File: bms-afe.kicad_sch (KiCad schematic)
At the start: 13 parts, among them J1 CONN HEADER VERT 7POS 2.5MM

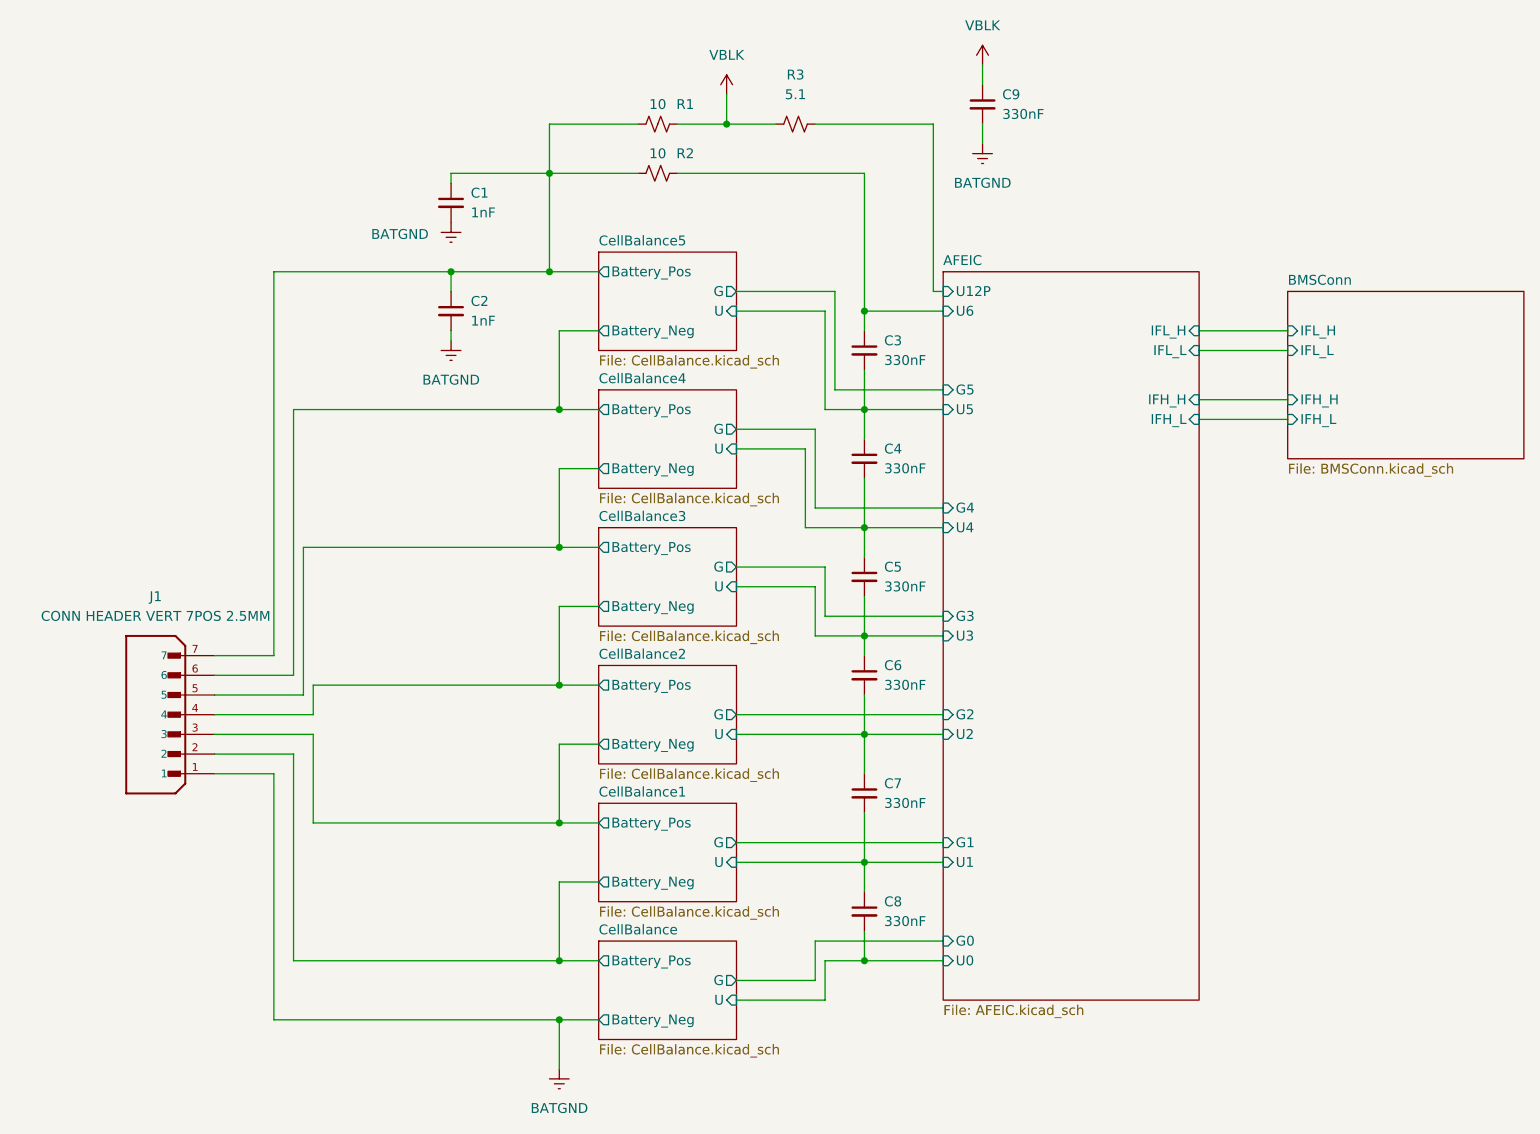
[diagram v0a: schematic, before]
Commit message: passive values
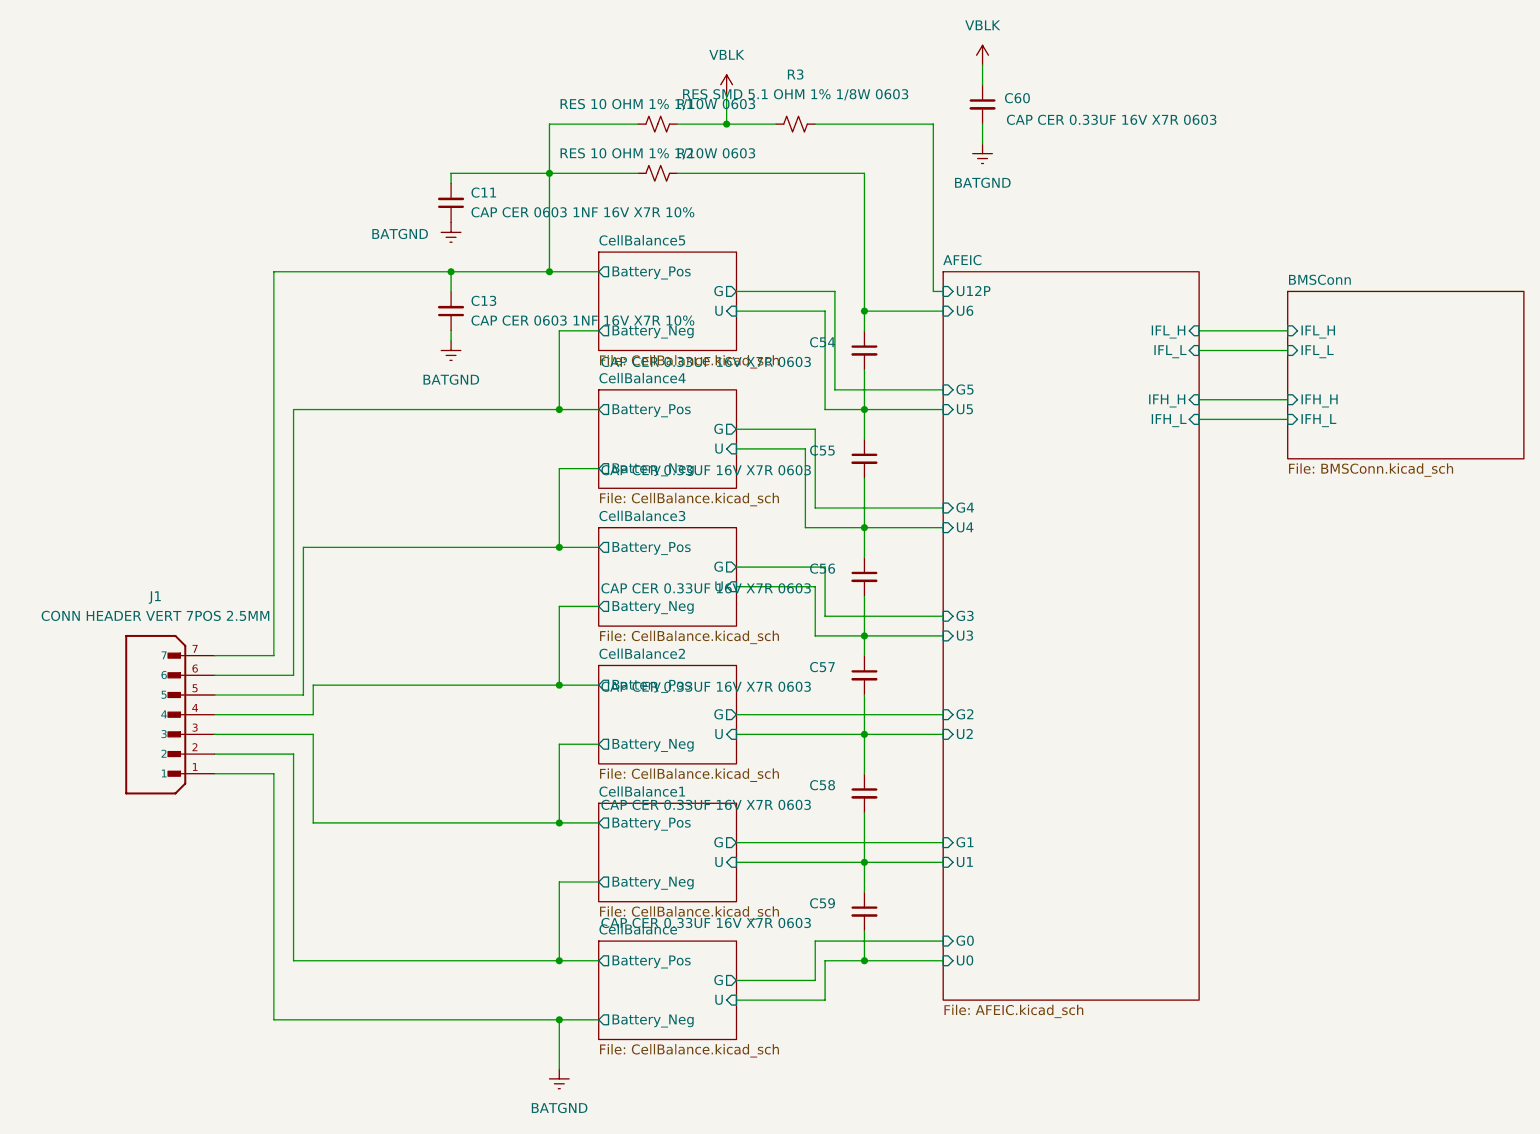
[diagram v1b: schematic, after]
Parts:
- removed C1, C2: 1nF, symbol Device:C_Small
- removed C3, C4, C5, C6, C7, C8, C9: 330nF, symbol Device:C_Small
- added C11, C13: CAP CER 0603 1NF 16V X7R 10%, Capacitor_SMD:C_0603_1608Metric, symbol Device:C_Small
- added C54, C55, C56, C57, C58, C59, C60: CAP CER 0.33UF 16V X7R 0603, Capacitor_SMD:C_0603_1608Metric, symbol Device:C_Small
- R1, R2: value 10 -> RES 10 OHM 1% 1/10W 0603; footprint (none) -> Resistor_SMD:R_0603_1608Metric
- R3: value 5.1 -> RES SMD 5.1 OHM 1% 1/8W 0603; footprint (none) -> Resistor_SMD:R_0603_1608Metric; LCSC (none) -> C242492
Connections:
- net AFEIC/U0: now also C59.2
- net AFEIC/U1: now also C58.2, C59.1
- net AFEIC/U2: now also C57.2, C58.1
- net AFEIC/U3: now also C56.2, C57.1
- net AFEIC/U4: now also C55.2, C56.1
- net AFEIC/U5: now also C54.2, C55.1
- net AFEIC/U6: now also C54.1
- net BATGND: now also C11.1, C13.1, C60.2
- net CellBalance5/Battery_Pos: now also C11.2, C13.2
- net VBLK: now also C60.1
